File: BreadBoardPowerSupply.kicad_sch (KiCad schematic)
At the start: 0 parts

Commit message: Make electronic schematic
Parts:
- added C1: 100nF, symbol Device:C
- added C3: 1uF, symbol Device:C_Polarized
- added D1_Green_LED1: LED, LED_THT:LED_D3.0mm, symbol Device:LED
- added D2: 1N4007, Diode_THT:D_DO-41_SOD81_P10.16mm_Horizontal, symbol Diode:1N4007
- added J1: Barrel_Jack, DCJ200-10-A-XX-K_REVA:GCT_DCJ200-10-A-XX-K_REVA, symbol MySymbols:DCJ200-10-A-XX-K_REVA
- added J2, J3: Conn_01x04_Pin, symbol Connector:Conn_01x04_Pin
- added J4, J5: Conn_01x02_Pin, symbol Connector:Conn_01x02_Pin
- added R1: 240R, symbol Device:R
- added R2: 2200, Resistor_THT:R_Axial_DIN0207_L6.3mm_D2.5mm_P10.16mm_Horizontal, symbol Device:R
- added RV1: 2000R, symbol Device:R_Potentiometer
- added S1: TL2285EE, TL2285EE, symbol MySymbols:TL2285EE
- added U1: Mini Digital Voltometer, symbol MySymbols:Mini Digital Voltometer
- added U2: LM317_TO-220, Package_TO_SOT_THT:TO-220-3_Vertical, symbol Regulator_Linear:LM317_TO-220
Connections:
- new net: D1_Green_LED1.2 (A), R2.2
- new net: R1.1, RV1.1, RV1.2, U2.1 (ADJ)
- new net: D2.2 (A), S1.2 (NO_1)
- new net +12V: J1.1, S1.3 (COMM_1), S1.4 (COMM_2)
- new net DC_IN: C1.1, D2.1 (K), U1.2 (VCC), U2.3 (VI)
- new net DC_OUT: C3.1, J2.1 (Pin_1), J2.2 (Pin_2), J2.3 (Pin_3), J2.4 (Pin_4), J4.1 (Pin_1), J5.1 (Pin_1), R1.2, U1.1 (Measure), U2.2 (VO)
- new net GND: C1.2, C3.2, D1_Green_LED1.1 (K), J1.2, J3.1 (Pin_1), J3.2 (Pin_2), J3.3 (Pin_3), J3.4 (Pin_4), J4.2 (Pin_2), J5.2 (Pin_2), RV1.3, U1.3 (GND)
- new net ON/OFF GREEN LED: R2.1, S1.5 (NO_2)
- no-connect marks 0 -> 2
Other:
- note added: "Back Side"
- note added: "DC Voltage Input"
- note added: "Front Side"
- note added: "Left"
- note added: "Right"
- note added: "Voltage Measure"
- note added: "Voltage Output"
- note added: "Voltage Regulator (LM317)"

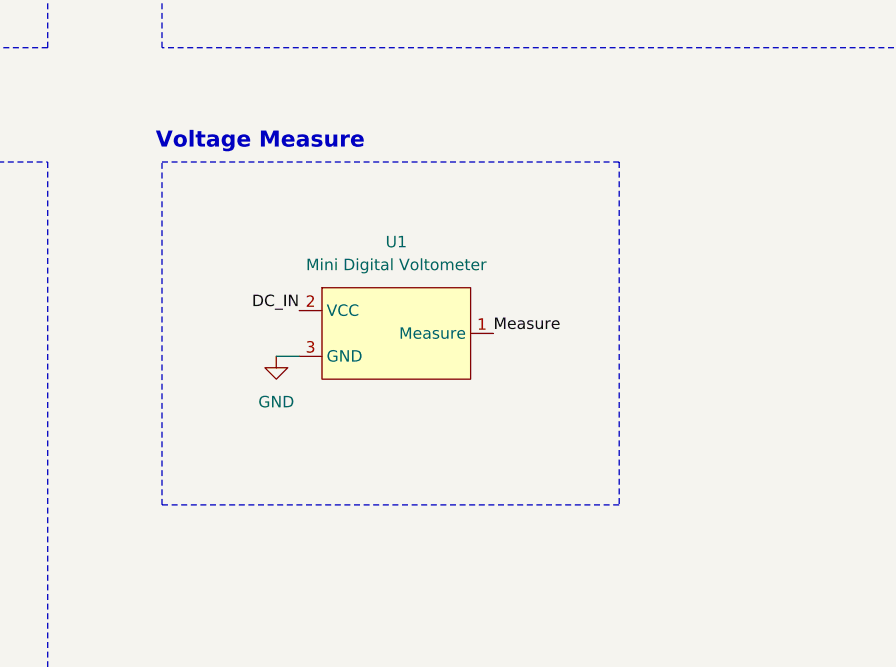
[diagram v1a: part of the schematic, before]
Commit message: Update electronics schematic
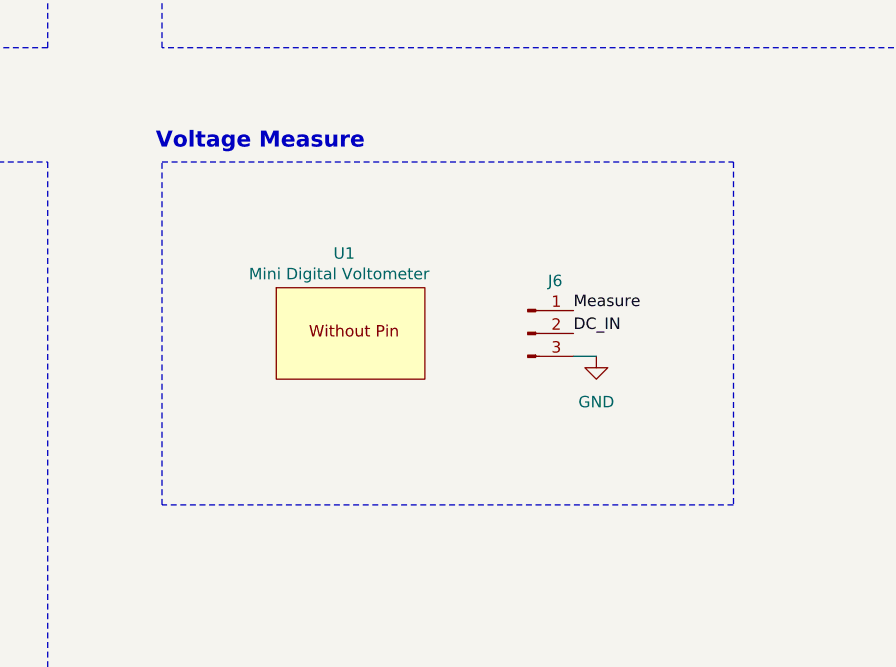
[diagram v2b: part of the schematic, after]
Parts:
- removed U1: Mini Digital Voltometer, symbol MySymbols:Mini Digital Voltometer
- added J6: Conn_01x03_Pin, symbol Connector:Conn_01x03_Pin
- added U1: Mini Digital Voltometer, symbol MySymbols:Mini Digital Voltometer Without Pin
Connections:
- net DC_IN: now also J6.2 (Pin_2)
- net DC_OUT: now also J6.1 (Pin_1)
- net GND: now also J6.3 (Pin_3)

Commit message: Update schematic and add footprint for symbols
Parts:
- C1, C3: footprint (none) -> Capacitor_SMD:C_0805_2012Metric_Pad1.18x1.45mm_HandSolder
- J1: footprint DCJ200-10-A-XX-K_REVA:GCT_DCJ200-10-A-XX-K_REVA -> MyFootPrints:GCT_DCJ200-10-A-XX-K_REVA
- J2, J3: footprint (none) -> Connector_PinHeader_2.54mm:PinHeader_1x04_P2.54mm_Vertical
- J4, J5: footprint (none) -> Connector_PinHeader_2.54mm:PinHeader_1x02_P2.54mm_Vertical
- J6: footprint (none) -> Connector_PinHeader_2.54mm:PinHeader_1x03_P2.54mm_Vertical
- R1: footprint (none) -> Resistor_SMD:R_0805_2012Metric_Pad1.20x1.40mm_HandSolder
- R2: footprint Resistor_THT:R_Axial_DIN0207_L6.3mm_D2.5mm_P10.16mm_Horizontal -> Resistor_SMD:R_0805_2012Metric_Pad1.20x1.40mm_HandSolder
- RV1: footprint (none) -> MyFootPrints:Potencjometr_WH148_3D
- S1: footprint TL2285EE -> MyFootPrints:TL2285EE
- U1: footprint (none) -> MyFootPrints:Mini_digital_voltmeter
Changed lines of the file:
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@@
 			)
 		)
-		(property "Footprint" ""
+		(property "Footprint" "Connector_PinHeader_2.54mm:PinHeader_1x04_P2.54mm_Vertical"
 			(at 180.34 63.5 0)
 			(hide yes)
@@
 			)
 		)
-		(property "Footprint" "Resistor_THT:R_Axial_DIN0207_L6.3mm_D2.5mm_P10.16mm_Horizontal"
+		(property "Footprint" "Resistor_SMD:R_0805_2012Metric_Pad1.20x1.40mm_HandSolder"
 			(at 88.9 80.518 90)
 			(hide yes)
@@
 			)
 		)
-		(property "Footprint" ""
+		(property "Footprint" "Resistor_SMD:R_0805_2012Metric_Pad1.20x1.40mm_HandSolder"
 			(at 85.09 135.128 90)
 			(hide yes)
@@
 			)
 		)
-		(property "Footprint" ""
+		(property "Footprint" "Connector_PinHeader_2.54mm:PinHeader_1x03_P2.54mm_Vertical"
 			(at 193.04 120.65 0)
 			(hide yes)
@@
 			)
 		)
-		(property "Footprint" ""
+		(property "Footprint" "Capacitor_SMD:C_0805_2012Metric_Pad1.18x1.45mm_HandSolder"
 			(at 56.8452 143.51 0)
 			(hide yes)
@@
 			)
 		)
-		(property "Footprint" "DCJ200-10-A-XX-K_REVA:GCT_DCJ200-10-A-XX-K_REVA"
+		(property "Footprint" "MyFootPrints:GCT_DCJ200-10-A-XX-K_REVA"
 			(at 35.56 60.96 0)
 			(hide yes)
@@
 			)
 		)
-		(property "Footprint" "TL2285EE"
+		(property "Footprint" "MyFootPrints:TL2285EE"
 			(at 114.3 150.8 0)
 			(hide yes)
@@
 			)
 		)
-		(property "Footprint" ""
+		(property "Footprint" "Capacitor_SMD:C_0805_2012Metric_Pad1.18x1.45mm_HandSolder"
 			(at 105.1052 143.51 0)
 			(hide yes)
@@
 			)
 		)
-		(property "Footprint" ""
+		(property "Footprint" "MyFootPrints:Mini_digital_voltmeter"
 			(at 173.99 120.65 0)
 			(hide yes)
@@
 			)
 		)
-		(property "Footprint" ""
+		(property "Footprint" "MyFootPrints:Potencjometr_WH148_3D"
 			(at 72.39 146.05 0)
 			(hide yes)
@@
 			)
 		)
-		(property "Footprint" ""
+		(property "Footprint" "Connector_PinHeader_2.54mm:PinHeader_1x02_P2.54mm_Vertical"
 			(at 208.28 63.5 0)
 			(hide yes)
@@
 			)
 		)
-		(property "Footprint" ""
+		(property "Footprint" "Connector_PinHeader_2.54mm:PinHeader_1x04_P2.54mm_Vertical"
 			(at 177.8 63.5 0)
 			(hide yes)
@@
 			)
 		)
-		(property "Footprint" ""
+		(property "Footprint" "Connector_PinHeader_2.54mm:PinHeader_1x02_P2.54mm_Vertical"
 			(at 226.06 63.5 0)
 			(hide yes)
